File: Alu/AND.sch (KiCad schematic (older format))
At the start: 4 parts, among them U5 74LS08, U6 74LS08

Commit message: footprints
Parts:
- C2, C3: footprint (none) -> Capacitor_SMD:C_0805_2012Metric
- U5, U6: footprint (none) -> Package_SO:SOIC-14_3.9x8.7mm_P1.27mm
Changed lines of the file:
@@
 $Descr A4 11693 8268
 encoding utf-8
-Sheet 2 156
+Sheet 2 191
 Title ""
 Date ""
@@
 F 0 "U5" V 1371 3770 50  0000 R CNN
 F 1 "74LS08" V 1280 3770 50  0000 R CNN
-F 2 "" H 1325 3950 50  0001 C CNN
+F 2 "Package_SO:SOIC-14_3.9x8.7mm_P1.27mm" H 1325 3950 50  0001 C CNN
 F 3 "http://www.ti.com/lit/gpn/sn74LS08" H 1325 3950 50  0001 C CNN
+F 4 "" H 0   0   50  0001 C CNN "Spice_Lib_File"
+F 5 "" H 0   0   50  0001 C CNN "Spice_Model"
+F 6 "" H 0   0   50  0001 C CNN "Spice_Netlist_Enabled"
+F 7 "" H 0   0   50  0001 C CNN "Spice_Primitive"
 	1    1325 3950
 	0    -1   -1   0
@@
 F 0 "U5" V 1971 3770 50  0000 R CNN
 F 1 "74LS08" V 1880 3770 50  0000 R CNN
-F 2 "" H 1925 3950 50  0001 C CNN
+F 2 "Package_SO:SOIC-14_3.9x8.7mm_P1.27mm" H 1925 3950 50  0001 C CNN
 F 3 "http://www.ti.com/lit/gpn/sn74LS08" H 1925 3950 50  0001 C CNN
+F 4 "" H 0   0   50  0001 C CNN "Spice_Lib_File"
+F 5 "" H 0   0   50  0001 C CNN "Spice_Model"
+F 6 "" H 0   0   50  0001 C CNN "Spice_Netlist_Enabled"
+F 7 "" H 0   0   50  0001 C CNN "Spice_Primitive"
 	2    1925 3950
 	0    -1   -1   0
@@
 F 0 "U5" V 2621 3695 50  0000 R CNN
 F 1 "74LS08" V 2530 3695 50  0000 R CNN
-F 2 "" H 2575 3875 50  0001 C CNN
+F 2 "Package_SO:SOIC-14_3.9x8.7mm_P1.27mm" H 2575 3875 50  0001 C CNN
 F 3 "http://www.ti.com/lit/gpn/sn74LS08" H 2575 3875 50  0001 C CNN
+F 4 "" H 0   0   50  0001 C CNN "Spice_Lib_File"
+F 5 "" H 0   0   50  0001 C CNN "Spice_Model"
+F 6 "" H 0   0   50  0001 C CNN "Spice_Netlist_Enabled"
+F 7 "" H 0   0   50  0001 C CNN "Spice_Primitive"
 	3    2575 3875
 	0    -1   -1   0
@@
 F 0 "U5" V 3346 3645 50  0000 R CNN
 F 1 "74LS08" V 3255 3645 50  0000 R CNN
-F 2 "" H 3300 3825 50  0001 C CNN
+F 2 "Package_SO:SOIC-14_3.9x8.7mm_P1.27mm" H 3300 3825 50  0001 C CNN
 F 3 "http://www.ti.com/lit/gpn/sn74LS08" H 3300 3825 50  0001 C CNN
+F 4 "" H 0   0   50  0001 C CNN "Spice_Lib_File"
+F 5 "" H 0   0   50  0001 C CNN "Spice_Model"
+F 6 "" H 0   0   50  0001 C CNN "Spice_Netlist_Enabled"
+F 7 "" H 0   0   50  0001 C CNN "Spice_Primitive"
 	4    3300 3825
 	0    -1   -1   0
@@
 F 0 "U6" H 9530 4471 50  0000 L CNN
 F 1 "74LS08" H 9530 4380 50  0000 L CNN
-F 2 "" H 9300 4425 50  0001 C CNN
+F 2 "Package_SO:SOIC-14_3.9x8.7mm_P1.27mm" H 9300 4425 50  0001 C CNN
 F 3 "http://www.ti.com/lit/gpn/sn74LS08" H 9300 4425 50  0001 C CNN
+F 4 "" H 0   0   50  0001 C CNN "Spice_Lib_File"
+F 5 "" H 0   0   50  0001 C CNN "Spice_Model"
+F 6 "" H 0   0   50  0001 C CNN "Spice_Netlist_Enabled"
+F 7 "" H 0   0   50  0001 C CNN "Spice_Primitive"
 	5    9300 4425
 	1    0    0    -1
-$EndComp
-$Comp
-L 74xx:74LS08 U6
-U 1 1 5FDB3B36
-P 3875 3950
-F 0 "U6" V 3921 3770 50  0000 R CNN
-F 1 "74LS08" V 3830 3770 50  0000 R CNN
-F 2 "" H 3875 3950 50  0001 C CNN
-F 3 "http://www.ti.com/lit/gpn/sn74LS08" H 3875 3950 50  0001 C CNN
-	1    3875 3950
-	0    -1   -1   0
 $EndComp
 $Comp
@@
 F 0 "U6" V 4521 3770 50  0000 R CNN
 F 1 "74LS08" V 4430 3770 50  0000 R CNN
-F 2 "" H 4475 3950 50  0001 C CNN
+F 2 "Package_SO:SOIC-14_3.9x8.7mm_P1.27mm" H 4475 3950 50  0001 C CNN
 F 3 "http://www.ti.com/lit/gpn/sn74LS08" H 4475 3950 50  0001 C CNN
+F 4 "" H 0   0   50  0001 C CNN "Spice_Lib_File"
+F 5 "" H 0   0   50  0001 C CNN "Spice_Model"
+F 6 "" H 0   0   50  0001 C CNN "Spice_Netlist_Enabled"
+F 7 "" H 0   0   50  0001 C CNN "Spice_Primitive"
 	2    4475 3950
 	0    -1   -1   0
@@
 F 0 "U6" V 5171 3695 50  0000 R CNN
 F 1 "74LS08" V 5080 3695 50  0000 R CNN
-F 2 "" H 5125 3875 50  0001 C CNN
+F 2 "Package_SO:SOIC-14_3.9x8.7mm_P1.27mm" H 5125 3875 50  0001 C CNN
 F 3 "http://www.ti.com/lit/gpn/sn74LS08" H 5125 3875 50  0001 C CNN
+F 4 "" H 0   0   50  0001 C CNN "Spice_Lib_File"
+F 5 "" H 0   0   50  0001 C CNN "Spice_Model"
+F 6 "" H 0   0   50  0001 C CNN "Spice_Netlist_Enabled"
+F 7 "" H 0   0   50  0001 C CNN "Spice_Primitive"
 	3    5125 3875
 	0    -1   -1   0
@@
 F 0 "U6" V 5896 3645 50  0000 R CNN
 F 1 "74LS08" V 5805 3645 50  0000 R CNN
-F 2 "" H 5850 3825 50  0001 C CNN
+F 2 "Package_SO:SOIC-14_3.9x8.7mm_P1.27mm" H 5850 3825 50  0001 C CNN
 F 3 "http://www.ti.com/lit/gpn/sn74LS08" H 5850 3825 50  0001 C CNN
+F 4 "" H 0   0   50  0001 C CNN "Spice_Lib_File"
+F 5 "" H 0   0   50  0001 C CNN "Spice_Model"
+F 6 "" H 0   0   50  0001 C CNN "Spice_Netlist_Enabled"
+F 7 "" H 0   0   50  0001 C CNN "Spice_Primitive"
 	4    5850 3825
 	0    -1   -1   0
@@
 F 0 "U5" H 8505 4496 50  0000 L CNN
 F 1 "74LS08" H 8505 4405 50  0000 L CNN
-F 2 "" H 8275 4450 50  0001 C CNN
+F 2 "Package_SO:SOIC-14_3.9x8.7mm_P1.27mm" H 8275 4450 50  0001 C CNN
 F 3 "http://www.ti.com/lit/gpn/sn74LS08" H 8275 4450 50  0001 C CNN
+F 4 "" H 0   0   50  0001 C CNN "Spice_Lib_File"
+F 5 "" H 0   0   50  0001 C CNN "Spice_Model"
+F 6 "" H 0   0   50  0001 C CNN "Spice_Netlist_Enabled"
+F 7 "" H 0   0   50  0001 C CNN "Spice_Primitive"
 	5    8275 4450
 	1    0    0    -1
@@
 F 0 "C2" H 7692 4571 50  0000 L CNN
 F 1 "100nF" H 7692 4480 50  0000 L CNN
-F 2 "" H 7600 4525 50  0001 C CNN
+F 2 "Capacitor_SMD:C_0805_2012Metric" H 7600 4525 50  0001 C CNN
 F 3 "~" H 7600 4525 50  0001 C CNN
+F 4 "" H 0   0   50  0001 C CNN "Spice_Lib_File"
+F 5 "" H 0   0   50  0001 C CNN "Spice_Model"
+F 6 "" H 0   0   50  0001 C CNN "Spice_Netlist_Enabled"
+F 7 "" H 0   0   50  0001 C CNN "Spice_Primitive"
 	1    7600 4525
 	1    0    0    -1
@@
 F 0 "C3" H 10092 4446 50  0000 L CNN
 F 1 "100nF" H 10092 4355 50  0000 L CNN
-F 2 "" H 10000 4400 50  0001 C CNN
+F 2 "Capacitor_SMD:C_0805_2012Metric" H 10000 4400 50  0001 C CNN
 F 3 "~" H 10000 4400 50  0001 C CNN
+F 4 "" H 0   0   50  0001 C CNN "Spice_Lib_File"
+F 5 "" H 0   0   50  0001 C CNN "Spice_Model"
+F 6 "" H 0   0   50  0001 C CNN "Spice_Netlist_Enabled"
+F 7 "" H 0   0   50  0001 C CNN "Spice_Primitive"
 	1    10000 4400
 	1    0    0    -1
@@
 Wire Wire Line
 	4775 2050 4775 2925
+$Comp
+L 74xx:74LS08 U6
+U 1 1 5CBB1308
+P 3875 3950
+F 0 "U6" V 3921 3770 50  0000 R CNN
+F 1 "74LS08" V 3830 3770 50  0000 R CNN
+F 2 "Package_SO:SOIC-14_3.9x8.7mm_P1.27mm" H 3875 3950 50  0001 C CNN
+F 3 "http://www.ti.com/lit/gpn/sn74LS08" H 3875 3950 50  0001 C CNN
+F 4 "" H 0   0   50  0001 C CNN "Spice_Lib_File"
+F 5 "" H 0   0   50  0001 C CNN "Spice_Model"
+F 6 "" H 0   0   50  0001 C CNN "Spice_Netlist_Enabled"
+F 7 "" H 0   0   50  0001 C CNN "Spice_Primitive"
+	1    3875 3950
+	0    -1   -1   0
+$EndComp
 $EndSCHEMATC

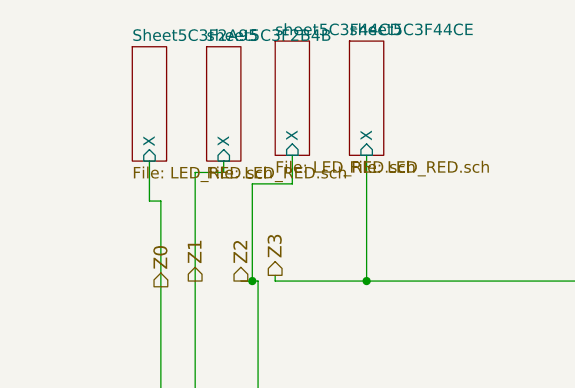
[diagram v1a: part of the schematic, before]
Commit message: started routing
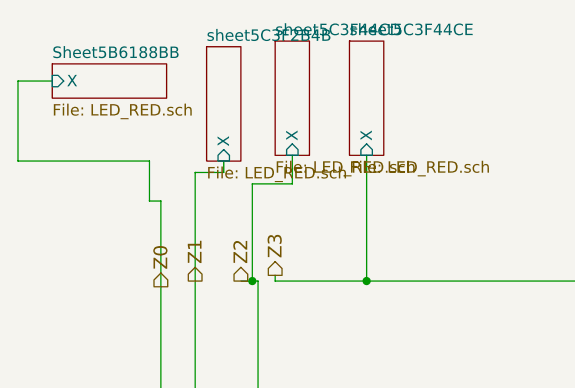
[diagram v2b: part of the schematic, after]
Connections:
- wire segments 109 -> 112
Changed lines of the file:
@@
 	9450 3925 9300 3925
-$Sheet
-S 1100 850  150  500
-U 5C3F2A96
-F0 "Sheet5C3F2A95" 50
-F1 "LED_RED.sch" 50
-F2 "X" I B 1175 1350 50
-$EndSheet
 $Sheet
 S 1425 850  150  500
@@
 	0    -1   -1   0
 $EndComp
+$Sheet
+S 750  925  500  150
+U 5B6188BC
+F0 "Sheet5B6188BB" 50
+F1 "LED_RED.sch" 50
+F2 "X" I L 750 1000 50
+$EndSheet
+Wire Wire Line
+	1175 1350 600  1350
+Wire Wire Line
+	600  1350 600  1000
+Wire Wire Line
+	600  1000 750  1000
 $EndSCHEMATC
